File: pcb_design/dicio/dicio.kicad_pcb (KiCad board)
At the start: 2 copper layers, 93 x 93 mm, 79 parts, among them J1 Conn_02x03_Counter_Clockwise, J2 Conn_01x06_Female, J3 USB_C_Receptacle, J4 Micro_SD_Card, J5 USB_C_Receptacle, J6 USB_C_Receptacle, J7 Conn_02x13_Odd_Even, J8 USB_C_Receptacle, Q1 Q_NMOS_GSD, SW1 SW_SPST, SW2 SW_SPST, U1 dsPIC33EP512MC806, U2 MCP2542FD, U3 S70FL01GS, U4 TPS737, U5 SiP32431, U6 SiP32431, U7 ADM7170, U8 FT232RL, Y1 Crystal_GND24, Y2 Crystal_GND24

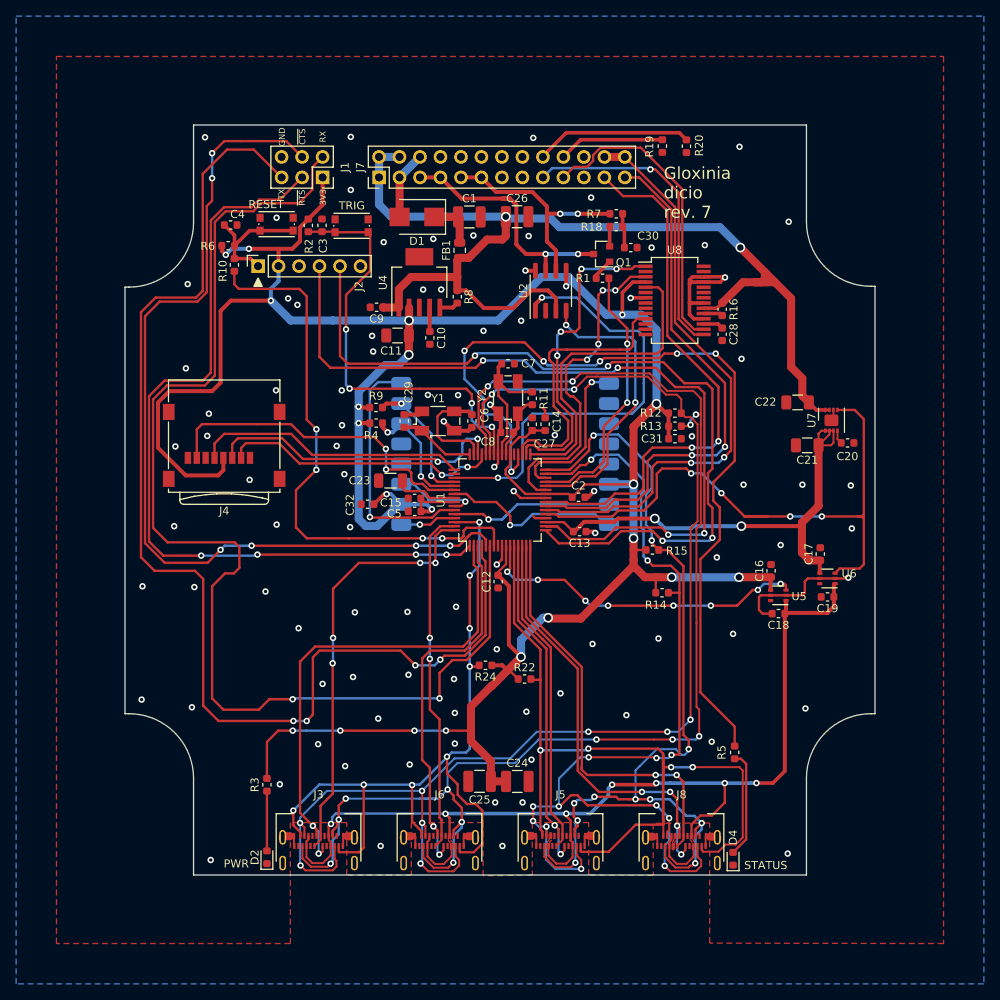
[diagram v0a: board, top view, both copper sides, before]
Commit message: New and updated board designs.
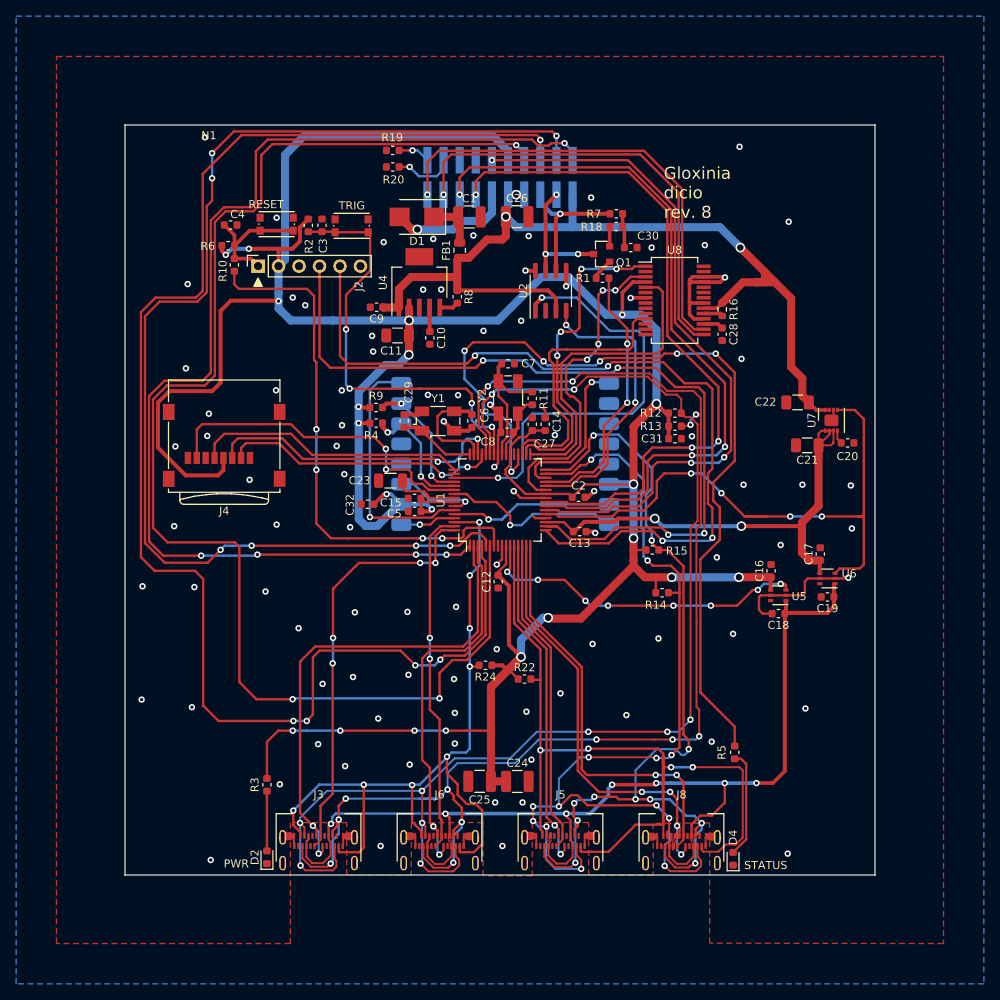
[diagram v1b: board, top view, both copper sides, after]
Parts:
- removed J7: Conn_02x13_Odd_Even, Connector_PinHeader_2.54mm:PinHeader_2x13_P2.54mm_Vertical
- J1: value Conn_02x03_Counter_Clockwise -> Conn_02x10_Odd_Even; footprint Connector_PinSocket_2.54mm:PinSocket_2x03_P2.54mm_Vertical -> samtec:SAMTEC_TMMH-110-01-T-DV; moved to B.Cu
- N1: footprint custom_footprints:Enclosure-Gloxinia2 -> custom_footprints:Enclosure-Gloxinia4
- R16: footprint Capacitor_SMD:C_0603_1608Metric -> Resistor_SMD:R_0603_1608Metric
- moved R20 36.5 mm to (71.7, 43.7), turned to 0 degrees
- moved R19 33.4 mm to (71.7, 41.6), turned to 180 degrees
- moved J1 22.0 mm to (85.0, 45.0), turned to 180 degrees
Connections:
- J1 pad 1: +3.3V -> VBUS
- J1 pad 2: /U1RX -> /~{U1RTS}
- J1 pad 3: /~{U1RTS} -> /CAN_H
- J1 pad 5: /U1TX -> /CAN_L
- J1 pad 6: GND -> /U1TX
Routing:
- net +3.3V: track 365.6 -> 410.1 mm
- net /~{U1RTS}: track 100.3 -> 141.5 mm, vias 4 -> 5
- net /~{U1CTS}: track 114.4 -> 148.8 mm, vias 6 -> 7
- net /U1TX: track 147.8 -> 182.1 mm, vias 4 -> 5
- net /CAN_C2: track 67.2 -> 90.8 mm, vias 2 -> 3
- net VBUS: track 135.5 -> 113.0 mm
- net /U1RX: track 146.6 -> 167.8 mm, vias 2 -> 3
- net /D-: track 38.0 -> 57.3 mm, vias 0 -> 1
- net /CAN_C1: track 67.8 -> 86.1 mm, vias 2 -> 3
- net /D+: track 38.1 -> 55.1 mm
- net /CAN_H: track 31.4 -> 16.0 mm, vias 2 -> 3
- net /SYNC: track 72.6 -> 86.4 mm, vias 2 -> 3
- net /CC1: track 19.5 -> 7.48 mm, vias 0 -> 1
- net /CAN_L: track 28.4 -> 17.5 mm, vias 2 -> 1
- net /VCONN: track 13.2 -> 4.02 mm, vias 0 -> 1
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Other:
- outline, holes or cut-outs redrawn
- board text added: "Gloxinia dicio rev. 8"
- board text removed: "3V3"
- board text removed: "GND"
- board text removed: "Gloxinia dicio rev. 7"
- board text removed: "RX"
- board text removed: "TX"
- board text removed: "~{CTS}"
- board text removed: "~{RTS}"
